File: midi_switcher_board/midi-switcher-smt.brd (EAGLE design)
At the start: 104.1 x 38.1 mm, 79 parts, among them IC1 6N138, IC2 PIC16F1825SO14, IC3 LD1086, Q1 MJD122GDPAK, Q2 MJD122GDPAK, Q3 MJD122GDPAK, Q4 MJD122GDPAK, Q5 MJD122GDPAK, Q6 MJD122GDPAK, Q7 MJD122GDPAK, Q8 MJD122GDPAK

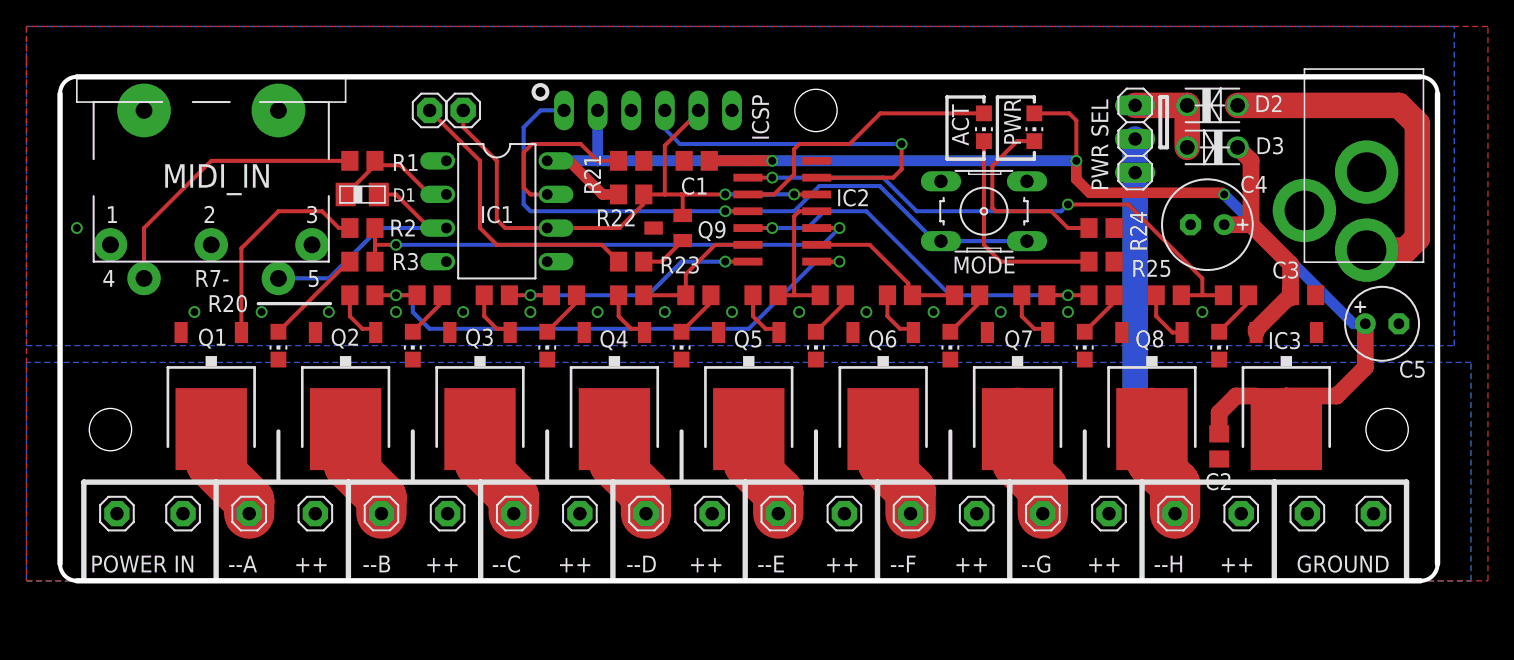
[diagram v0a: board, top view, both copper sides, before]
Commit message: pcb updates rev2
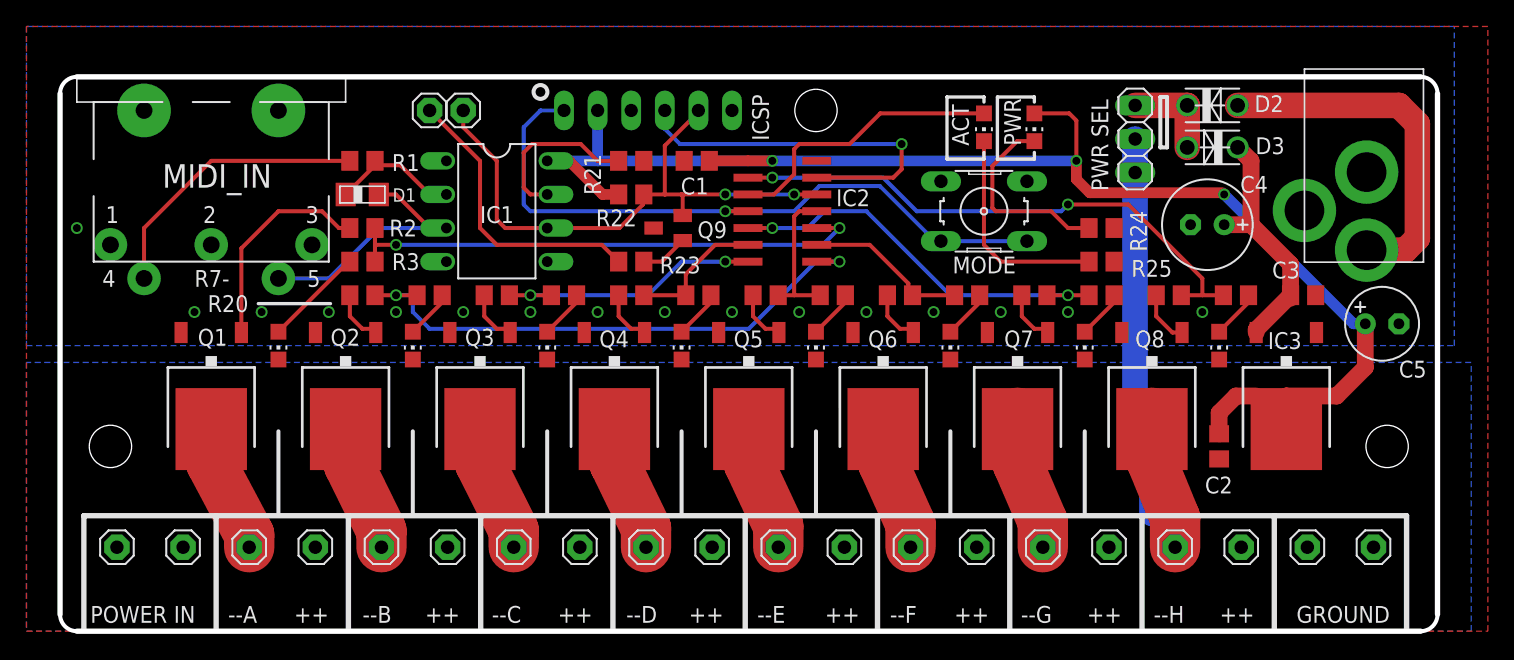
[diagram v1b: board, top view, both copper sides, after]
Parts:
- moved OP1+ 2.54 mm to (32.0, 5.08)
- moved OP1- 2.54 mm to (97.0, 5.08)
- moved OP2+ 2.54 mm to (102.0, 5.08)
- moved OP2- 2.54 mm to (87.0, 5.08)
- moved OP3+ 2.54 mm to (92.0, 5.08)
- moved OP3- 2.54 mm to (77.0, 5.08)
- moved OP4+ 2.54 mm to (82.0, 5.08)
- moved OP4- 2.54 mm to (67.0, 5.08)
- moved OP5+ 2.54 mm to (72.0, 5.08)
- moved OP5- 2.54 mm to (57.0, 5.08)
- moved OP6- 2.54 mm to (47.0, 5.08)
- moved OP7+ 2.54 mm to (52.0, 5.08)
- moved OP7- 2.54 mm to (37.0, 5.08)
- moved OP8+ 2.54 mm to (42.0, 5.08)
- moved OP8+1 2.54 mm to (62.0, 5.08)
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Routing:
- net +12V: track 26.3 -> 28.8 mm
- net N$25: track 8.34 -> 10.5 mm
- net N$26: track 8.41 -> 10.6 mm
- net N$27: track 7.25 -> 9.37 mm
- net N$31: track 7.31 -> 9.43 mm
- net N$29: track 7.38 -> 9.48 mm
- net N$42: track 7.51 -> 9.61 mm
- net N$30: track 7.45 -> 9.53 mm
- net N$47: track 7.58 -> 9.64 mm
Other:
- board size 104.1 x 38.1 mm -> 104.1 x 41.9 mm
- board text added: "Mini Module REV2"
- board text removed: "REV7"
